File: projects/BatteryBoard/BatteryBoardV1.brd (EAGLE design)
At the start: 87 x 92 mm, 213 parts, among them M1 BSO201SP, SW1 BTS50015-1TAD, SW2 BTS50015-1TAD, U1 LTC4412MPS6, U3 LTC4121, U4 LTC4121, U5 LTC4121, U6 LTC4121

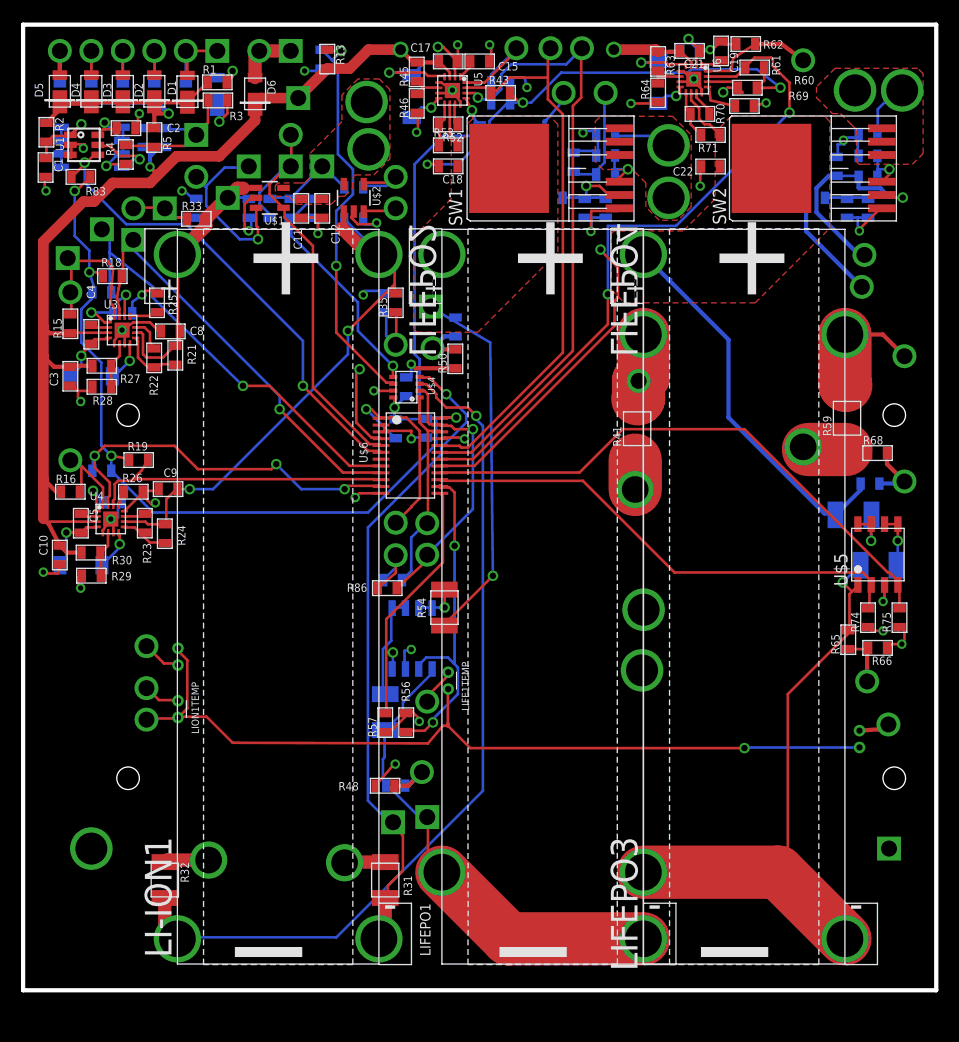
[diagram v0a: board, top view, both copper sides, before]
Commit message: Finished second round of Battery Board Layout
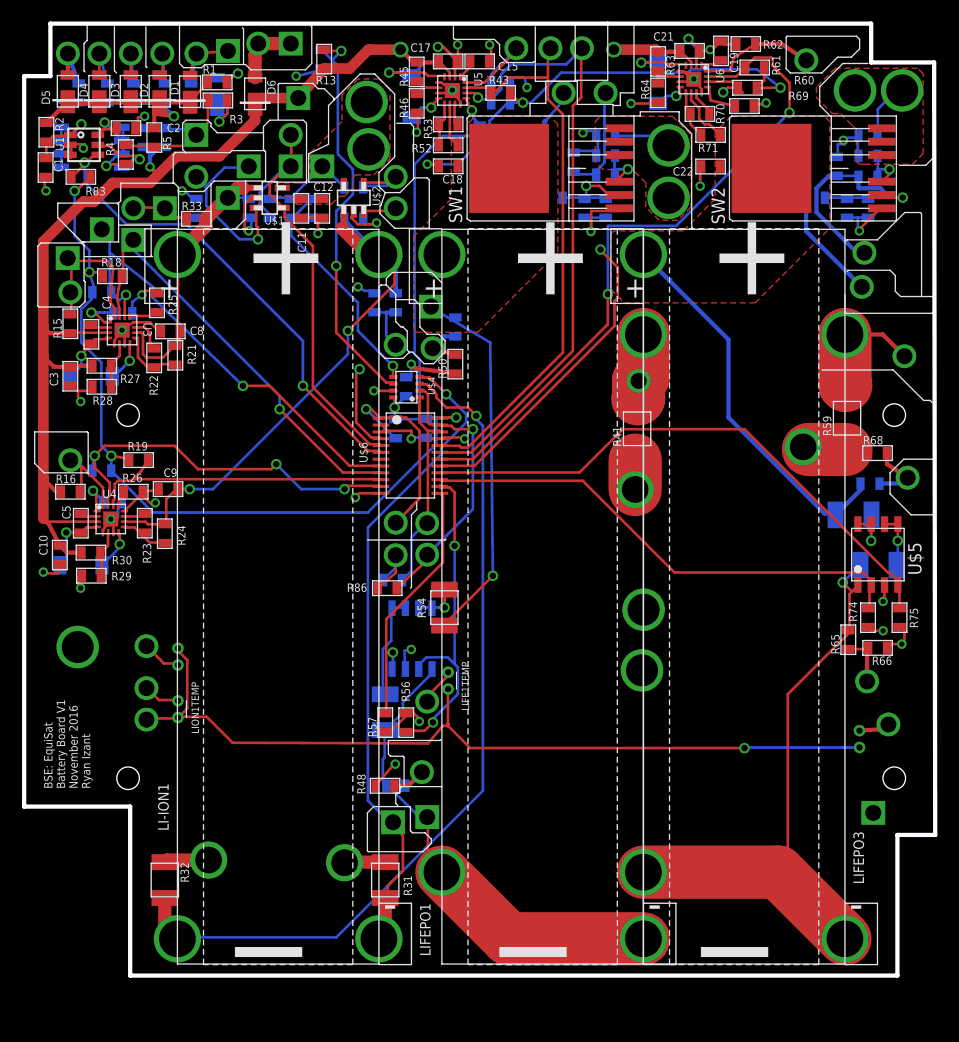
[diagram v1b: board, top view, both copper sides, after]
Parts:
- moved V13 19.2 mm to (-1.30, 30.2), turned to 90 degrees
- moved V12 3.72 mm to (74.5, 14.4)
- moved R10 1.78 mm to (-1.22, 83.0)
- moved R9 1.52 mm to (1.52, 83.0)
- moved V2 1.05 mm to (10.0, 86.7)
- moved R7 1.02 mm to (7.02, 83.0)
- moved R8 1.02 mm to (4.02, 83.0)
- moved V49 1.02 mm to (13.0, 87.0)
- moved R36 1.02 mm to (27.0, 63.0)
- moved V4 0.80 mm to (3.76, 86.7)
- moved V5 0.80 mm to (0.76, 86.7)
- moved V6 0.80 mm to (-2.24, 86.7)
- moved V3 0.80 mm to (6.76, 86.7)
- moved D3 0.76 mm to (3.76, 83.3)
- moved D4 0.76 mm to (0.76, 83.3)
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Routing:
- net SP_C: track 43.0 -> 47.9 mm
- net LION2: track 53.4 -> 56.9 mm
- net L2_REF: track 6.72 -> 5.55 mm
- net GND: track 185.8 -> 186.6 mm
- net UMB_CHG: track 5.71 -> 6.38 mm
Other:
- board size 87 x 92 mm -> 86.8 x 90.7 mm
- board text added: "BSE: EquiSat Battery Board V1 November 2016 Ryan Izant"
